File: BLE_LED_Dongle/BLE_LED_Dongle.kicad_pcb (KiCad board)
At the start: 2 copper layers, 98.6 x 61.2 mm, 188 parts, among them J1 Conn_01x04, J2 Conn_02x08_Counter_Clockwise, J3 USB_C_Receptacle_PowerOnly_6P, SW1 SW_SPDT, U1 nRF52810-QCxx, U2 TPS61023DRLR, U3 TP4056-42-ESOP8, U4 XC6206PxxxMR, Y1 Crystal, Y2 Crystal_GND23

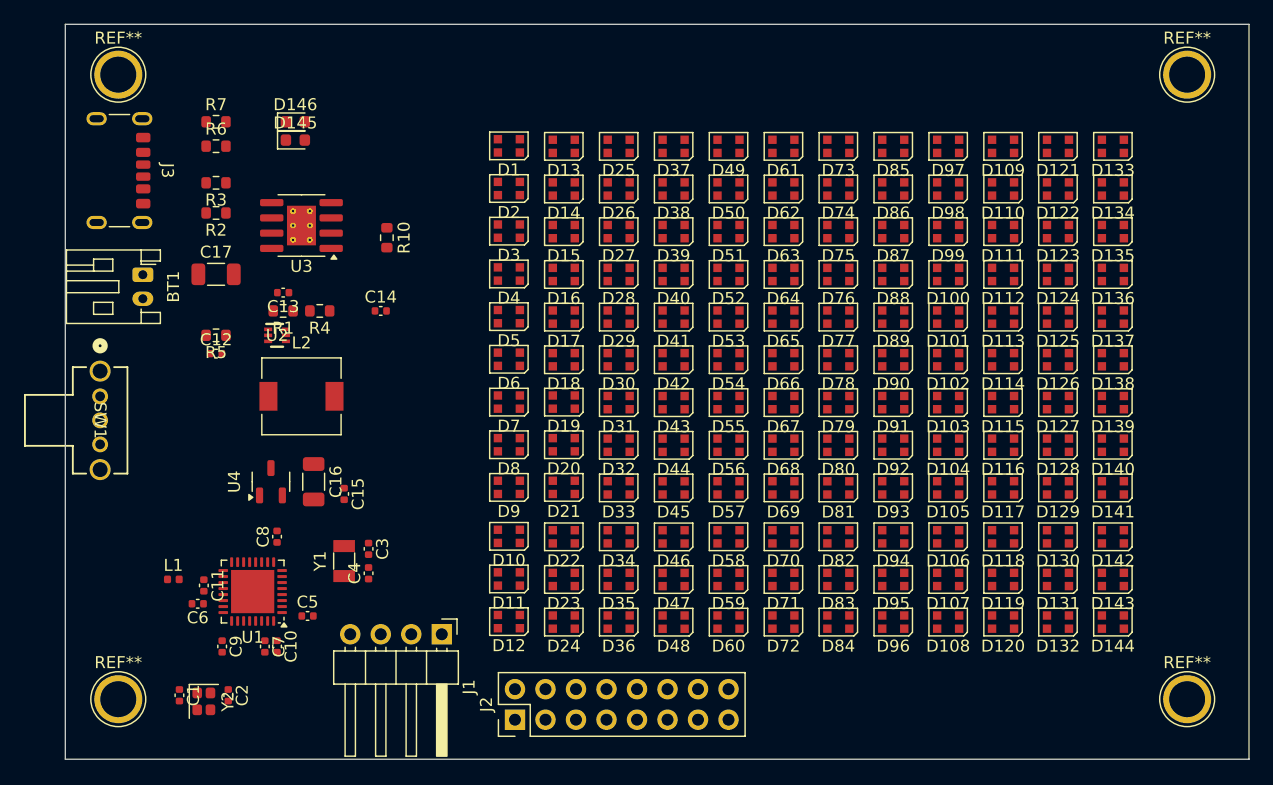
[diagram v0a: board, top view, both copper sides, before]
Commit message: progress: board 1 complete, board 2 schematics in progress.
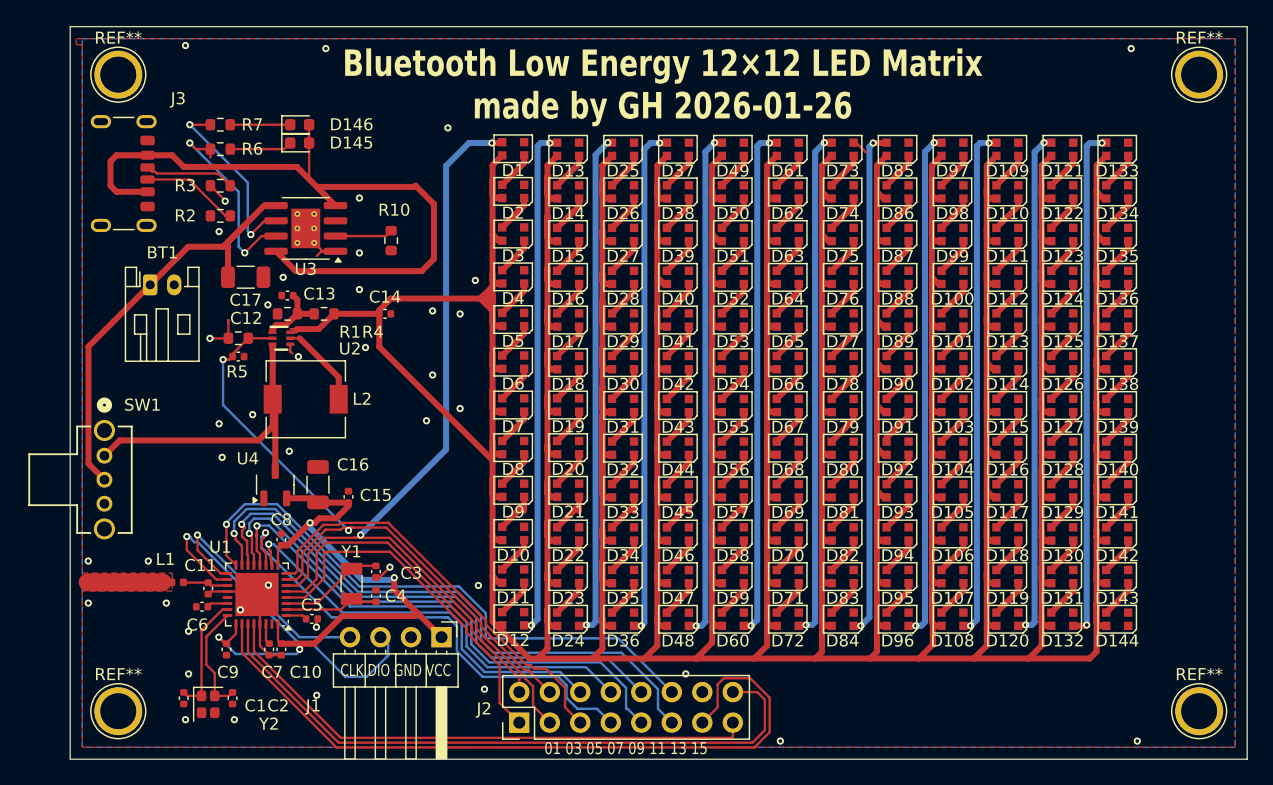
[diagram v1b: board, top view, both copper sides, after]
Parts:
- removed the REF** at (185.0, 23.0)
- removed the REF** at (185.0, 75.0)
- removed the REF** at (96.0, 75.0)
- added REF**: TestPoint_Plated_Hole_D3.0mm, TestPoint:TestPoint_Plated_Hole_D3.0mm, F.Cu at (186.0, 23.0)
- added REF**: TestPoint_Plated_Hole_D3.0mm, TestPoint:TestPoint_Plated_Hole_D3.0mm, F.Cu at (186.0, 76.0)
- added REF**: TestPoint_Plated_Hole_D3.0mm, TestPoint:TestPoint_Plated_Hole_D3.0mm, F.Cu at (96.0, 76.0)
- moved SW1 4.95 mm to (94.8, 54.7)
- moved C17 2.48 mm to (106.6, 39.9), turned to 180 degrees
- moved C4 1.99 mm to (117.5, 66.4)
- moved Y1 1.99 mm to (115.4, 65.4)
- moved C3 1.99 mm to (117.5, 64.4)
- moved R5 1.87 mm to (106.0, 44.9)
- moved C12 1.87 mm to (106.0, 46.5)
- moved BT1 1.04 mm to (98.7, 40.5), turned to 0 degrees
- moved D101 0.43 mm to (165.5, 43.4)
- moved D102 0.43 mm to (165.5, 47.0)
- moved D104 0.43 mm to (165.5, 54.1)
- moved D110 0.43 mm to (170.0, 32.8)
- moved D111 0.43 mm to (170.0, 36.3)
- moved D113 0.43 mm to (170.0, 43.4)
- moved D114 0.43 mm to (170.0, 47.0)
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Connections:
- J2 pad 10: unconnected-(J2-Pin_10-Pad10) -> Net-(J2-Pin_12)
- J2 pad 11: Net-(J2-Pin_11) -> Net-(J2-Pin_6)
- J2 pad 12: Net-(J2-Pin_12) -> Net-(J2-Pin_11)
- J2 pad 13: Net-(J2-Pin_13) -> Net-(J2-Pin_7)
- J2 pad 14: Net-(J2-Pin_14) -> unconnected-(J2-Pin_10-Pad14)
- J2 pad 15: /Power/EN_5V -> Net-(J2-Pin_8)
- J2 pad 16: Net-(J2-Pin_16) -> Net-(U1-P0.28/AIN4)
- J2 pad 2: /LED_Matrix1/DIN -> Net-(J2-Pin_16)
- J2 pad 3: Net-(J2-Pin_3) -> /LED_Matrix1/DIN
- J2 pad 4: Net-(J2-Pin_4) -> /Power/EN_5V
- J2 pad 5: Net-(J2-Pin_5) -> Net-(J2-Pin_3)
- J2 pad 6: Net-(J2-Pin_6) -> Net-(J2-Pin_14)
- J2 pad 7: Net-(J2-Pin_7) -> Net-(J2-Pin_4)
- J2 pad 8: Net-(J2-Pin_8) -> Net-(J2-Pin_13)
- J2 pad 9: Net-(J2-Pin_9) -> Net-(J2-Pin_5)
- U1 pad 27: Net-(J2-Pin_9) -> Net-(U1-P0.28/AIN4)
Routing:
- net +5V: track 0.00 -> 815.3 mm
- net /LED_Matrix1/DIN: track 0.00 -> 72.1 mm, vias 0 -> 2
- net Vusb: track 0.00 -> 62.9 mm
- net Net-(J2-Pin_7): track 0.00 -> 61.9 mm
- net +3.3V: track 0.00 -> 55.7 mm, vias 0 -> 4
- net /Power/EN_5V: track 0.00 -> 54.7 mm, vias 0 -> 2
- net Net-(U1-P0.28/AIN4): track 0.00 -> 54.4 mm
- net Net-(J2-Pin_6): track 0.00 -> 50.3 mm, vias 0 -> 1
- net Net-(J2-Pin_11): track 0.00 -> 49.3 mm, vias 0 -> 1
- net Net-(J2-Pin_8): track 0.00 -> 46.4 mm
- net Net-(J2-Pin_5): track 0.00 -> 45.7 mm, vias 0 -> 1
- net Net-(J2-Pin_12): track 0.00 -> 44.9 mm, vias 0 -> 1
- net /LED_Matrix1/LED_Matrix_Line10/DOUT: track 0.00 -> 42.8 mm, vias 0 -> 2
- net /LED_Matrix1/LED_Matrix_Line4/DOUT: track 0.00 -> 42.5 mm, vias 0 -> 2
- net /LED_Matrix1/LED_Matrix_Line8/DOUT: track 0.00 -> 42.5 mm, vias 0 -> 2
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- added copper zone on B.Cu, net GND
- added copper zone on F.Cu, net GND
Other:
- board size 98.6 x 61.2 mm -> 98 x 61 mm
- board text added: "01 03 05 07 09 11 13 15"
- board text added: "Bluetooth Low Energy 12×12 LED Matrix made by GH 2026-01-26"
- board text added: "CLK DIO GND VCC"
